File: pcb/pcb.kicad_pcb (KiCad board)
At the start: 2 copper layers, 100 x 88.7 mm, 65 parts, among them J1 AudioJack4, J2 USB_C_Receptacle_USB2.0, SW1 Switch, SW10 Switch, SW11 Switch, SW12 Switch, SW13 Switch, SW14 Switch, SW15 Switch, SW16 Switch, SW17 Switch, SW18 Switch, SW2 Switch, SW3 Switch, SW4 Switch, SW5 Switch, SW6 Switch, SW7 Switch, SW8 Switch, SW9 Switch, U1 MCU_rp2040-zero, U2 MCU_rp2040-zero, U3 RollerEncoder_EVQWGD001

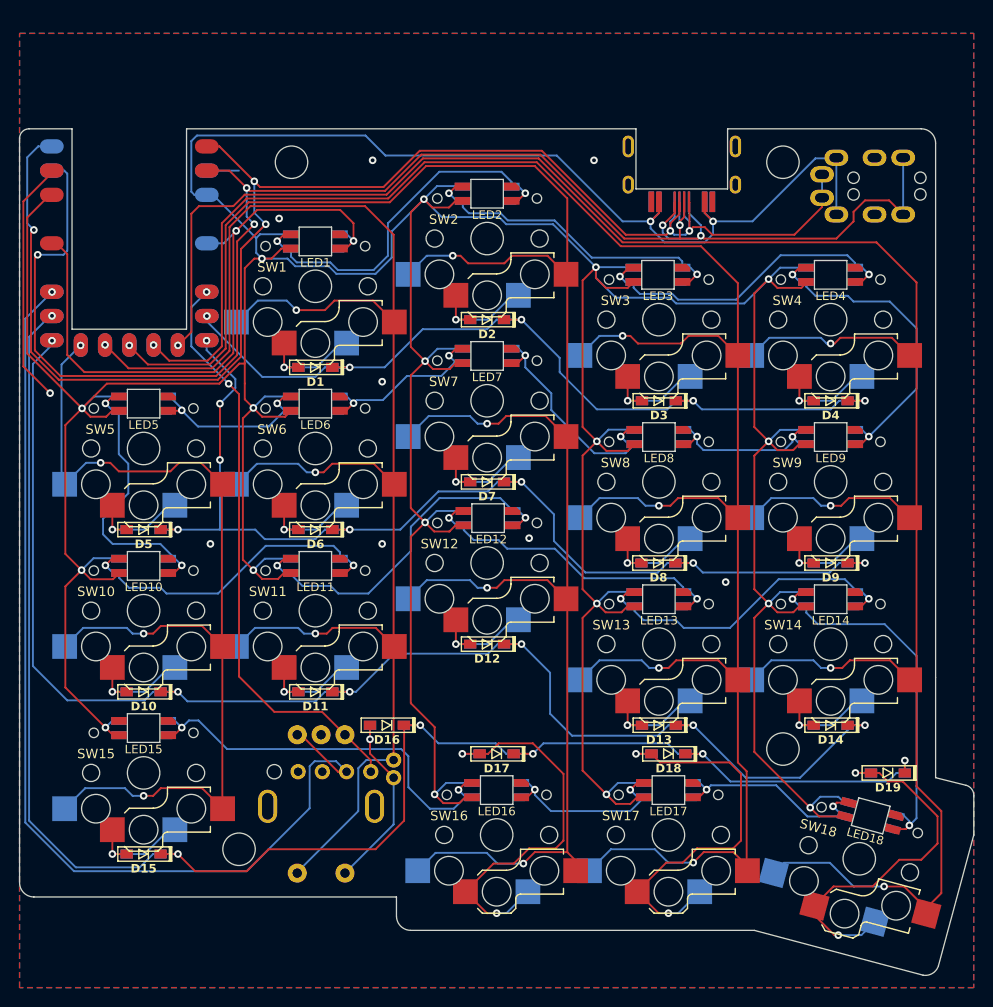
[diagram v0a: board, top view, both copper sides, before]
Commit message: v2
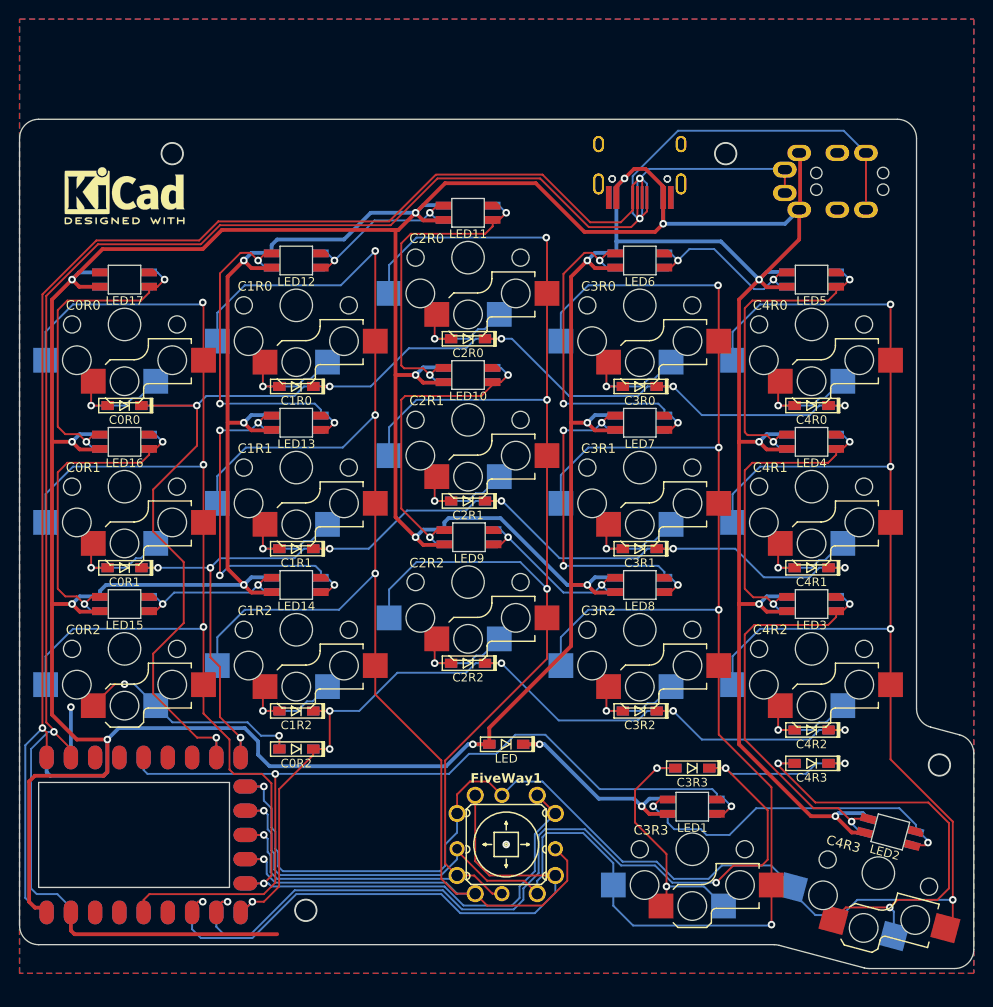
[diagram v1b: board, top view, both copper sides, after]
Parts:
- removed the D17 at (102.5, 106.0)
- removed D19: D_Small, zzkeeb:Diode_1N4148-SOD123-reversible-flip3d
- removed H1, H2, H3, H4: MountingHole, zzkeeb:Hole_M2-spacer
- removed J2: USB_C_Receptacle_USB2.0, zzkeeb:Connector_USB-C-mid-mount-ali-reversible-data
- removed the LED16 at (102.5, 109.8)
- removed RE1: RotaryEncoder_Switch, zzkeeb:RotaryEncoder_EC11-reversible
- removed the SW16 at (102.5, 114.5)
- removed U3: RollerEncoder_EVQWGD001, zzkeeb:RotaryEncoder_EVQWGD001
- added D18: Diode, zzkeeb:Diode_1N4148-SOD123-reversible-flip3d, B.Cu at (103.5, 105.0)
- added FiveWay1: 5Way-Tactile_K1-1506DN-01, zzkeeb:Button_5way-reversible, F.Cu at (103.5, 115.5)
- added REF**: KiCad-Logo2_5mm_SilkScreen, Symbol:KiCad-Logo2_5mm_SilkScreen, F.Cu at (63.5, 47.5)
- added REF**: Logo_QMK-silkscreen, zzkeeb:Logo_QMK-silkscreen, B.Cu at (63.5, 47.5)
- added Ref**: Val**, zzkeeb:Hole_M2, F.Cu at (68.5, 43.1)
- added Ref**: Val**, zzkeeb:Hole_M2, F.Cu at (126.5, 43.1)
- added Ref**: Val**, zzkeeb:Hole_M2, F.Cu at (148.9, 107.2)
- added Ref**: Val**, zzkeeb:Hole_M2, F.Cu at (82.5, 122.4)
- added USB1: Connector_HRO-TYPE-C-31-M-12, zzkeeb:Connector_HRO-TYPE-C-31-M-12-data, F.Cu at (117.5, 39.5)
- added USB2: Connector_HRO-TYPE-C-31-M-12, zzkeeb:Connector_HRO-TYPE-C-31-M-12-data, B.Cu at (117.5, 39.5)
- D1: renamed from D5; value D_Small -> Diode
- D10: renamed from D9; value D_Small -> Diode
- D11: renamed from D15; value D_Small -> Diode
- D12: renamed from D11; value D_Small -> Diode
- D13: renamed from D12; value D_Small -> Diode
- D14: renamed from D13; value D_Small -> Diode
- D15: renamed from D14; value D_Small -> Diode
- D16: renamed from D18; value D_Small -> Diode
- D17: renamed from D16; value D_Small -> Diode
- D2: renamed from D1; value D_Small -> Diode
- D3: renamed from D2; value D_Small -> Diode
- D4: renamed from D3; value D_Small -> Diode
- D5: renamed from D4; value D_Small -> Diode
- D6: renamed from D10; value D_Small -> Diode
- D7: renamed from D6; value D_Small -> Diode
- D8: renamed from D7; value D_Small -> Diode
- D9: renamed from D8; value D_Small -> Diode
- LED1: renamed from LED17; footprint zzkeeb:LED_SK6812-MINI-E-reversible -> zzkeeb:LED_SK6812-MINI-E-reversible-flip3d
- LED10: renamed from LED7; footprint zzkeeb:LED_SK6812-MINI-E-reversible -> zzkeeb:LED_SK6812-MINI-E-reversible-flip3d
- LED11: renamed from LED2; footprint zzkeeb:LED_SK6812-MINI-E-reversible -> zzkeeb:LED_SK6812-MINI-E-reversible-flip3d
- LED12: renamed from LED1; footprint zzkeeb:LED_SK6812-MINI-E-reversible -> zzkeeb:LED_SK6812-MINI-E-reversible-flip3d
- LED13: renamed from LED6; footprint zzkeeb:LED_SK6812-MINI-E-reversible -> zzkeeb:LED_SK6812-MINI-E-reversible-flip3d
- LED14: renamed from LED11; footprint zzkeeb:LED_SK6812-MINI-E-reversible -> zzkeeb:LED_SK6812-MINI-E-reversible-flip3d
- LED15: footprint zzkeeb:LED_SK6812-MINI-E-reversible -> zzkeeb:LED_SK6812-MINI-E-reversible-flip3d
- LED16: renamed from LED10; footprint zzkeeb:LED_SK6812-MINI-E-reversible -> zzkeeb:LED_SK6812-MINI-E-reversible-flip3d
- LED17: renamed from LED5; footprint zzkeeb:LED_SK6812-MINI-E-reversible -> zzkeeb:LED_SK6812-MINI-E-reversible-flip3d
- LED2: renamed from LED18; footprint zzkeeb:LED_SK6812-MINI-E-reversible -> zzkeeb:LED_SK6812-MINI-E-reversible-flip3d
- LED3: renamed from LED14; footprint zzkeeb:LED_SK6812-MINI-E-reversible -> zzkeeb:LED_SK6812-MINI-E-reversible-flip3d
- LED4: renamed from LED9; footprint zzkeeb:LED_SK6812-MINI-E-reversible -> zzkeeb:LED_SK6812-MINI-E-reversible-flip3d
- LED5: renamed from LED4; footprint zzkeeb:LED_SK6812-MINI-E-reversible -> zzkeeb:LED_SK6812-MINI-E-reversible-flip3d
- LED6: renamed from LED3; footprint zzkeeb:LED_SK6812-MINI-E-reversible -> zzkeeb:LED_SK6812-MINI-E-reversible-flip3d
- LED7: renamed from LED8; footprint zzkeeb:LED_SK6812-MINI-E-reversible -> zzkeeb:LED_SK6812-MINI-E-reversible-flip3d
- LED8: renamed from LED13; footprint zzkeeb:LED_SK6812-MINI-E-reversible -> zzkeeb:LED_SK6812-MINI-E-reversible-flip3d
- LED9: renamed from LED12; footprint zzkeeb:LED_SK6812-MINI-E-reversible -> zzkeeb:LED_SK6812-MINI-E-reversible-flip3d
- moved U1 62.0 mm to (65.5, 114.5), turned to -90 degrees
- moved U2 62.0 mm to (65.5, 114.5), turned to 90 degrees
- moved D17 44.7 mm to (135.5, 107.0)
- moved D11 19.4 mm to (81.5, 105.5)
- moved D1 13.2 mm to (63.5, 69.5)
- moved D6 13.2 mm to (63.5, 86.5)
- moved LED15 13.2 mm to (63.5, 90.3)
- moved LED16 13.2 mm to (63.5, 73.3)
- moved LED17 13.2 mm to (63.5, 56.3)
- moved SW1 13.2 mm to (63.5, 61.0)
- moved SW11 13.2 mm to (63.5, 95.0)
- moved SW6 13.2 mm to (63.5, 78.0)
- moved J1 3.93 mm to (144.5, 46.0)
- moved LED1 3.04 mm to (123.0, 111.5)
- moved D16 2.92 mm to (123.0, 107.5)
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- renumbered SW5 to SW1, SW9 to SW10, SW15 to SW11, SW11 to SW12, SW12 to SW13, SW13 to SW14, SW14 to SW15, SW17 to SW16, SW18 to SW17, SW1 to SW2, SW2 to SW3, SW3 to SW4, SW4 to SW5, SW10 to SW6, SW6 to SW7, SW7 to SW8, SW8 to SW9
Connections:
- net ENCB renamed row4
- D1 pad 1: row1 -> row0
- D11 pad 1: row3 -> row2
- D17 pad 2: SW_ENCA -> Net-(D17-A)
- D6 pad 1: row2 -> row1
- J1 pad T: VCC -> +5V
- LED1 pad 1: VCC -> Net-(D18-K)
- LED1 pad 2: Net-(LED16-Pad4) -> Net-(LED1-DOUT)
- LED1 pad 4: Net-(LED17-Pad4) -> LED
- LED10 pad 1: VCC -> +5V
- LED10 pad 2: Net-(LED6-Pad4) -> Net-(LED10-DOUT)
- LED10 pad 4: Net-(LED7-Pad4) -> Net-(LED10-DIN)
- LED11 pad 1: VCC -> +5V
- LED11 pad 2: Net-(LED2-Pad2) -> Net-(LED11-DOUT)
- LED11 pad 4: Net-(LED1-Pad2) -> Net-(LED10-DOUT)
- LED12 pad 1: VCC -> +5V
- LED12 pad 2: Net-(LED1-Pad2) -> Net-(LED12-DOUT)
- LED12 pad 4: LED -> Net-(LED11-DOUT)
- LED13 pad 1: VCC -> +5V
- LED13 pad 2: Net-(LED5-Pad4) -> Net-(LED13-DOUT)
- LED13 pad 4: Net-(LED6-Pad4) -> Net-(LED12-DOUT)
- LED14 pad 1: VCC -> +5V
- LED14 pad 2: Net-(LED11-Pad2) -> Net-(LED14-DOUT)
- LED14 pad 4: Net-(LED10-Pad2) -> Net-(LED13-DOUT)
- LED15 pad 1: VCC -> +5V
- LED15 pad 2: unconnected-(LED15-Pad2) -> Net-(LED15-DOUT)
- LED15 pad 4: Net-(LED15-Pad4) -> Net-(LED14-DOUT)
- LED16 pad 1: VCC -> +5V
- LED16 pad 2: Net-(LED10-Pad2) -> Net-(LED16-DOUT)
- LED16 pad 4: Net-(LED10-Pad4) -> Net-(LED15-DOUT)
- LED17 pad 1: VCC -> +5V
- LED17 pad 2: Net-(LED10-Pad4) -> unconnected-(LED17-DOUT-Pad2)
- LED17 pad 4: Net-(LED5-Pad4) -> Net-(LED16-DOUT)
- LED2 pad 1: VCC -> +5V
- LED2 pad 2: Net-(LED17-Pad4) -> Net-(LED2-DOUT)
- LED2 pad 4: Net-(LED14-Pad2) -> Net-(LED1-DOUT)
- LED3 pad 1: VCC -> +5V
- LED3 pad 2: Net-(LED14-Pad2) -> Net-(LED3-DOUT)
- LED3 pad 4: Net-(LED13-Pad2) -> Net-(LED2-DOUT)
- LED4 pad 1: VCC -> +5V
- LED4 pad 2: Net-(LED8-Pad4) -> Net-(LED4-DOUT)
- LED4 pad 4: Net-(LED4-Pad2) -> Net-(LED3-DOUT)
- LED5 pad 1: VCC -> +5V
- LED5 pad 2: Net-(LED4-Pad2) -> Net-(LED5-DOUT)
- LED5 pad 4: Net-(LED3-Pad2) -> Net-(LED4-DOUT)
- LED6 pad 1: VCC -> +5V
- LED6 pad 2: Net-(LED3-Pad2) -> Net-(LED6-DOUT)
- LED6 pad 4: Net-(LED2-Pad2) -> Net-(LED5-DOUT)
- LED7 pad 1: VCC -> +5V
- LED7 pad 2: Net-(LED7-Pad4) -> Net-(LED7-DOUT)
- LED7 pad 4: Net-(LED8-Pad4) -> Net-(LED6-DOUT)
- LED8 pad 1: VCC -> +5V
- LED8 pad 2: Net-(LED13-Pad2) -> Net-(LED8-DOUT)
- LED8 pad 4: Net-(LED12-Pad2) -> Net-(LED7-DOUT)
- LED9 pad 1: VCC -> +5V
- LED9 pad 2: Net-(LED12-Pad2) -> Net-(LED10-DIN)
- LED9 pad 4: Net-(LED11-Pad2) -> Net-(LED8-DOUT)
- SW17 pad 1: Net-(D19-Pad2) -> Net-(D17-A)
- U1 pad 17: ENCA -> unconnected-(U1-26-Pad17)
- U1 pad 21: VCC -> unconnected-(U1-3V3-Pad21)
- U2 pad 21: VCC -> unconnected-(U2-3V3-Pad21)
- U2 pad 7: ENCA -> unconnected-(U2-6-Pad7)
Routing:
- net VCC: track 635.8 -> 0.00 mm, vias 20 -> 0
- net +5V: track 0.00 -> 633.9 mm, vias 0 -> 20
- net row3: track 175.1 -> 105.3 mm, vias 6 -> 4
- net col0: track 106.6 -> 174.3 mm
- net ENCA: track 61.7 -> 0.00 mm, vias 2 -> 0
- net row2: track 149.7 -> 99.0 mm
- net row0: track 93.6 -> 142.3 mm, vias 5 -> 6
- net Net-(D17-A): track 0.00 -> 47.5 mm, vias 0 -> 2
- net Net-(LED15-Pad4): track 44.0 -> 0.00 mm, vias 2 -> 0
- net Net-(LED2-DOUT): track 0.00 -> 44.0 mm, vias 0 -> 2
- net row4: track 107.1 -> 64.8 mm
- net Net-(D17-Pad2): track 42.1 -> 0.00 mm, vias 2 -> 0
- net col2: track 210.1 -> 169.6 mm, vias 5 -> 4
- net Net-(LED14-Pad2): track 39.7 -> 0.00 mm, vias 2 -> 0
- net Net-(D19-Pad2): track 39.3 -> 0.00 mm, vias 2 -> 0
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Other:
- board size 100 x 88.7 mm -> 100 x 89 mm
- board text added: "v2.0"
- board text removed: "v1.1"
